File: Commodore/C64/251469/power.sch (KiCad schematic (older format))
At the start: 21 parts, among them CN10 LED Connector, CN7 Power Input, SW1 Power Switch

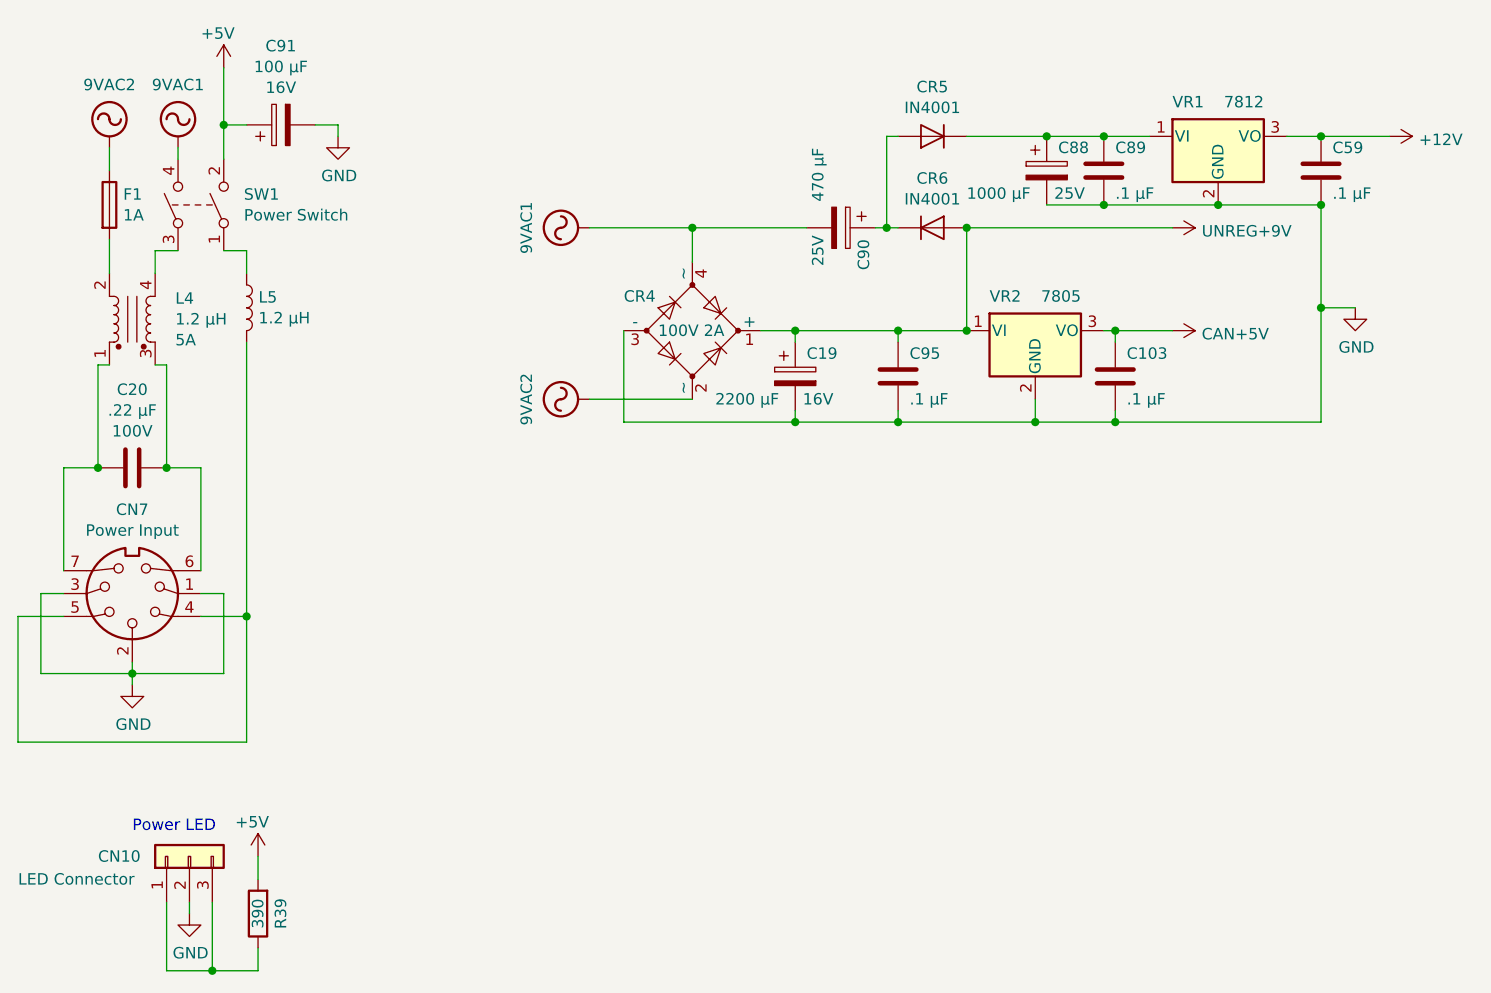
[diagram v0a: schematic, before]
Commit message: Tweaks
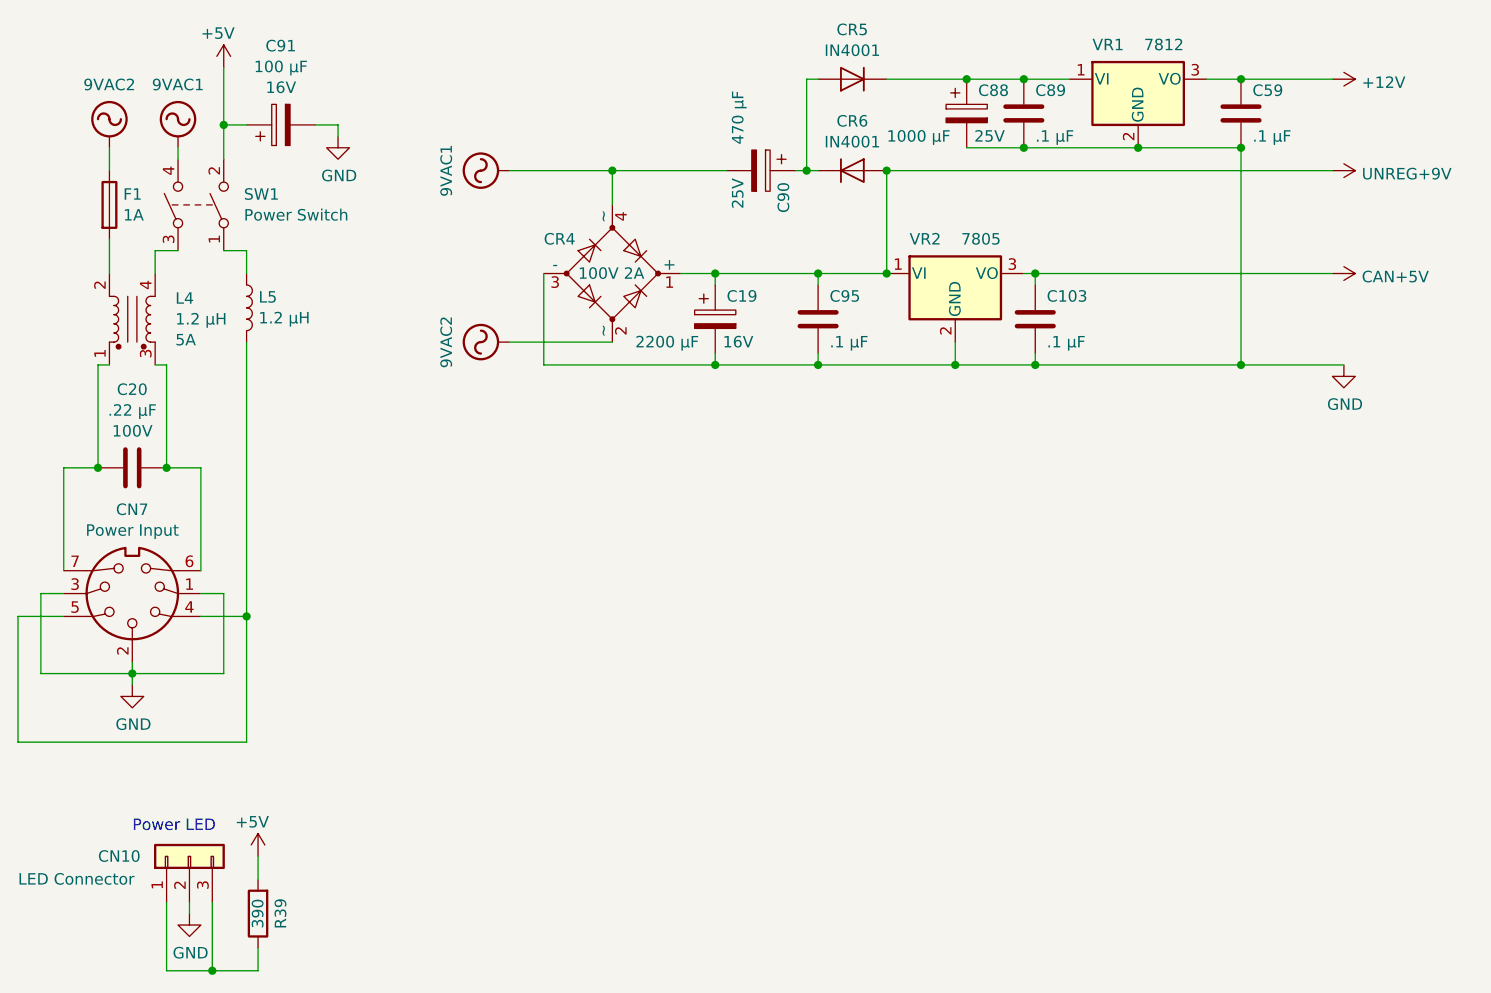
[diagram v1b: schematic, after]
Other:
- moved on the sheet: C103, C19, C59, C88, C89, C90, C95, CR4, CR5, CR6, VR1, VR2
